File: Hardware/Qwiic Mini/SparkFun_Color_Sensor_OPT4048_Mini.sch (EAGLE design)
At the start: 26 parts, among them J4 QWIIC_RIGHT_ANGLE, J5 QWIIC_RIGHT_ANGLE, U1 OPT4048

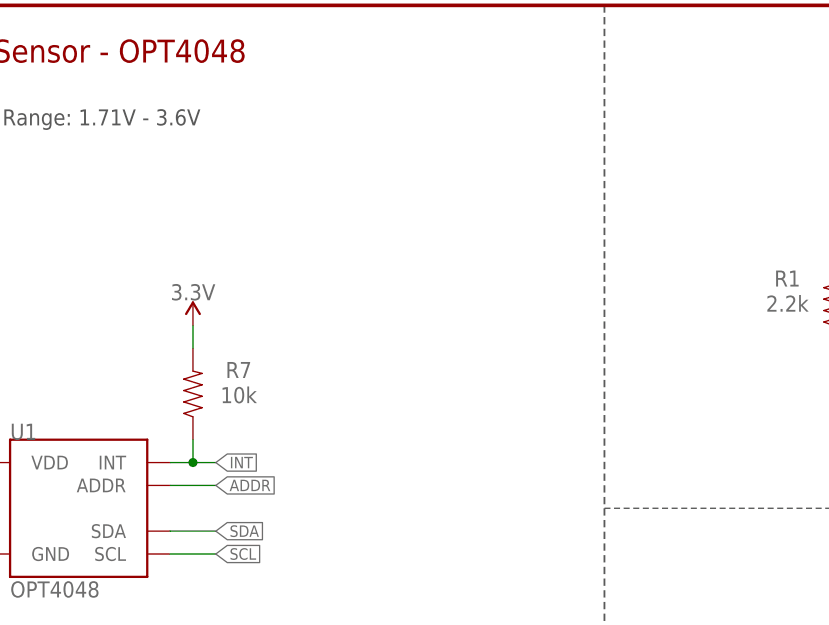
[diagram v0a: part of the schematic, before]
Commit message: Adds jumper to interrupt pin on both designs
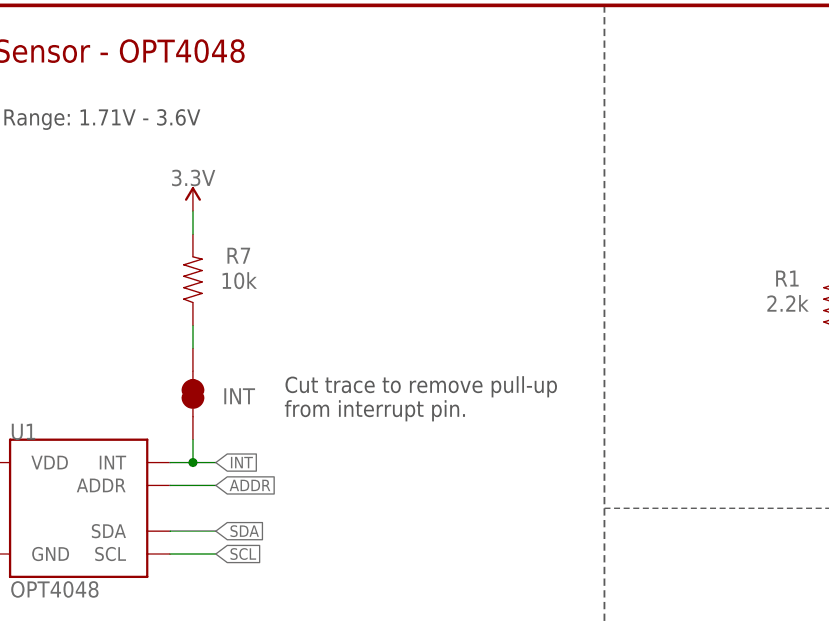
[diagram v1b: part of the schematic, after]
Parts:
- added INT: JUMPER-SMT_2_NC_TRACE_SILK, SparkFun-Jumpers:JUMPER-SMT_2_NC_TRACE_SILK
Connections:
- new net N$5: INT.2, R7.1
- net INT: now also INT.1; no longer R7.1
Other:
- note added: "Cut trace to remove pull-up from interrupt pin."
- moved on the sheet: R7
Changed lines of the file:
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@@
 <part name="0X45" library="SparkFun-Jumpers" deviceset="JUMPER-SMT_2_NO" device="_SILK" package3d_urn="urn:adsk.eagle:package:39279/1"/>
 <part name="0X44" library="SparkFun-Jumpers" deviceset="JUMPER-SMT_2_NC_TRACE" device="_SILK" package3d_urn="urn:adsk.eagle:package:39281/1"/>
+<part name="INT" library="SparkFun-Jumpers" deviceset="JUMPER-SMT_2_NC_TRACE" device="_SILK" package3d_urn="urn:adsk.eagle:package:39281/1"/>
 </parts>
 <sheets>
@@
 <text x="177.8" y="116.84" size="1.778" layer="97" font="vector" align="center">Close Jumper to select
 respective Address.</text>
+<text x="78.74" y="139.7" size="1.778" layer="97" font="vector">Cut trace to remove pull-up
+from interrupt pin. </text>
 </plain>
 <instances>
@@
 <attribute name="VALUE" x="43.18" y="119.126" size="1.778" layer="96" font="vector" align="top-center"/>
 </instance>
-<instance part="R7" gate="G$1" x="68.58" y="142.24" smashed="yes" rot="R90">
-<attribute name="NAME" x="73.66" y="145.796" size="1.778" layer="95" font="vector" rot="R180" align="bottom-center"/>
-<attribute name="VALUE" x="73.66" y="141.224" size="1.778" layer="96" font="vector" rot="R180" align="top-center"/>
-</instance>
-<instance part="SUPPLY11" gate="G$1" x="68.58" y="149.86" smashed="yes">
-<attribute name="VALUE" x="68.58" y="152.654" size="1.778" layer="96" font="vector" align="bottom-center"/>
+<instance part="R7" gate="G$1" x="68.58" y="154.94" smashed="yes" rot="R90">
+<attribute name="NAME" x="73.66" y="158.496" size="1.778" layer="95" font="vector" rot="R180" align="bottom-center"/>
+<attribute name="VALUE" x="73.66" y="153.924" size="1.778" layer="96" font="vector" rot="R180" align="top-center"/>
+</instance>
+<instance part="SUPPLY11" gate="G$1" x="68.58" y="162.56" smashed="yes">
+<attribute name="VALUE" x="68.58" y="165.354" size="1.778" layer="96" font="vector" align="bottom-center"/>
 </instance>
 <instance part="SUPPLY12" gate="G$1" x="147.32" y="116.84" smashed="yes">
@@
 <instance part="0X44" gate="G$1" x="139.7" y="86.36" smashed="yes">
 <attribute name="NAME" x="139.7" y="89.154" size="1.778" layer="95" font="vector" align="center"/>
+</instance>
+<instance part="INT" gate="G$1" x="68.58" y="142.24" smashed="yes" rot="R90">
+<attribute name="NAME" x="73.66" y="141.986" size="1.778" layer="95" font="vector" rot="R180" align="center"/>
 </instance>
 </instances>
@@
 <segment>
 <pinref part="R7" gate="G$1" pin="2"/>
-<wire x1="68.58" y1="149.86" x2="68.58" y2="147.32" width="0.1524" layer="91"/>
+<wire x1="68.58" y1="162.56" x2="68.58" y2="160.02" width="0.1524" layer="91"/>
 <pinref part="SUPPLY11" gate="G$1" pin="3.3V"/>
 </segment>
@@
 <segment>
 <pinref part="U1" gate="G$1" pin="INT"/>
-<wire x1="68.58" y1="134.62" x2="66.04" y2="134.62" width="0.1524" layer="91"/>
+<label x="71.12" y="134.62" size="1.27" layer="95" font="vector" xref="yes"/>
+<wire x1="66.04" y1="134.62" x2="68.58" y2="134.62" width="0.1524" layer="91"/>
+<pinref part="INT" gate="G$1" pin="1"/>
+<wire x1="68.58" y1="134.62" x2="71.12" y2="134.62" width="0.1524" layer="91"/>
 <wire x1="68.58" y1="137.16" x2="68.58" y2="134.62" width="0.1524" layer="91"/>
-<pinref part="R7" gate="G$1" pin="1"/>
-<label x="71.12" y="134.62" size="1.27" layer="95" font="vector" xref="yes"/>
-<wire x1="68.58" y1="134.62" x2="71.12" y2="134.62" width="0.1524" layer="91"/>
 <junction x="68.58" y="134.62"/>
 </segment>
@@
 </segment>
 </net>
+<net name="N$5" class="0">
+<segment>
+<pinref part="INT" gate="G$1" pin="2"/>
+<pinref part="R7" gate="G$1" pin="1"/>
+<wire x1="68.58" y1="147.32" x2="68.58" y2="149.86" width="0.1524" layer="91"/>
+</segment>
+</net>

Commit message: Revert "Adds jumper to interrupt pin on both designs"
This reverts commit a39334068ad88ec2875ce3e39fad74091b9d5839.
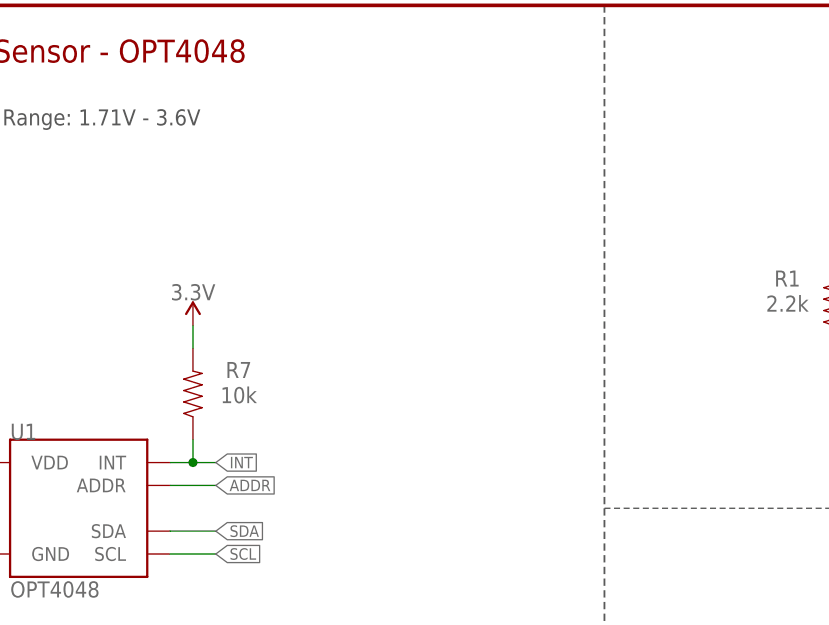
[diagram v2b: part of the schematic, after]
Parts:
- removed INT: JUMPER-SMT_2_NC_TRACE_SILK, SparkFun-Jumpers:JUMPER-SMT_2_NC_TRACE_SILK
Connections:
- removed net N$5: INT.2, R7.1
- net INT: now also R7.1; no longer INT.1
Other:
- note removed: "Cut trace to remove pull-up from interrupt pin."
- moved on the sheet: R7
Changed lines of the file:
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@@
 <part name="0X45" library="SparkFun-Jumpers" deviceset="JUMPER-SMT_2_NO" device="_SILK" package3d_urn="urn:adsk.eagle:package:39279/1"/>
 <part name="0X44" library="SparkFun-Jumpers" deviceset="JUMPER-SMT_2_NC_TRACE" device="_SILK" package3d_urn="urn:adsk.eagle:package:39281/1"/>
-<part name="INT" library="SparkFun-Jumpers" deviceset="JUMPER-SMT_2_NC_TRACE" device="_SILK" package3d_urn="urn:adsk.eagle:package:39281/1"/>
 </parts>
 <sheets>
@@
 <text x="177.8" y="116.84" size="1.778" layer="97" font="vector" align="center">Close Jumper to select
 respective Address.</text>
-<text x="78.74" y="139.7" size="1.778" layer="97" font="vector">Cut trace to remove pull-up
-from interrupt pin. </text>
 </plain>
 <instances>
@@
 <attribute name="VALUE" x="43.18" y="119.126" size="1.778" layer="96" font="vector" align="top-center"/>
 </instance>
-<instance part="R7" gate="G$1" x="68.58" y="154.94" smashed="yes" rot="R90">
-<attribute name="NAME" x="73.66" y="158.496" size="1.778" layer="95" font="vector" rot="R180" align="bottom-center"/>
-<attribute name="VALUE" x="73.66" y="153.924" size="1.778" layer="96" font="vector" rot="R180" align="top-center"/>
-</instance>
-<instance part="SUPPLY11" gate="G$1" x="68.58" y="162.56" smashed="yes">
-<attribute name="VALUE" x="68.58" y="165.354" size="1.778" layer="96" font="vector" align="bottom-center"/>
+<instance part="R7" gate="G$1" x="68.58" y="142.24" smashed="yes" rot="R90">
+<attribute name="NAME" x="73.66" y="145.796" size="1.778" layer="95" font="vector" rot="R180" align="bottom-center"/>
+<attribute name="VALUE" x="73.66" y="141.224" size="1.778" layer="96" font="vector" rot="R180" align="top-center"/>
+</instance>
+<instance part="SUPPLY11" gate="G$1" x="68.58" y="149.86" smashed="yes">
+<attribute name="VALUE" x="68.58" y="152.654" size="1.778" layer="96" font="vector" align="bottom-center"/>
 </instance>
 <instance part="SUPPLY12" gate="G$1" x="147.32" y="116.84" smashed="yes">
@@
 <instance part="0X44" gate="G$1" x="139.7" y="86.36" smashed="yes">
 <attribute name="NAME" x="139.7" y="89.154" size="1.778" layer="95" font="vector" align="center"/>
-</instance>
-<instance part="INT" gate="G$1" x="68.58" y="142.24" smashed="yes" rot="R90">
-<attribute name="NAME" x="73.66" y="141.986" size="1.778" layer="95" font="vector" rot="R180" align="center"/>
 </instance>
 </instances>
@@
 <segment>
 <pinref part="R7" gate="G$1" pin="2"/>
-<wire x1="68.58" y1="162.56" x2="68.58" y2="160.02" width="0.1524" layer="91"/>
+<wire x1="68.58" y1="149.86" x2="68.58" y2="147.32" width="0.1524" layer="91"/>
 <pinref part="SUPPLY11" gate="G$1" pin="3.3V"/>
 </segment>
@@
 <segment>
 <pinref part="U1" gate="G$1" pin="INT"/>
+<wire x1="68.58" y1="134.62" x2="66.04" y2="134.62" width="0.1524" layer="91"/>
+<wire x1="68.58" y1="137.16" x2="68.58" y2="134.62" width="0.1524" layer="91"/>
+<pinref part="R7" gate="G$1" pin="1"/>
 <label x="71.12" y="134.62" size="1.27" layer="95" font="vector" xref="yes"/>
-<wire x1="66.04" y1="134.62" x2="68.58" y2="134.62" width="0.1524" layer="91"/>
-<pinref part="INT" gate="G$1" pin="1"/>
 <wire x1="68.58" y1="134.62" x2="71.12" y2="134.62" width="0.1524" layer="91"/>
-<wire x1="68.58" y1="137.16" x2="68.58" y2="134.62" width="0.1524" layer="91"/>
 <junction x="68.58" y="134.62"/>
 </segment>
@@
 </segment>
 </net>
-<net name="N$5" class="0">
-<segment>
-<pinref part="INT" gate="G$1" pin="2"/>
-<pinref part="R7" gate="G$1" pin="1"/>
-<wire x1="68.58" y1="147.32" x2="68.58" y2="149.86" width="0.1524" layer="91"/>
-</segment>
-</net>
